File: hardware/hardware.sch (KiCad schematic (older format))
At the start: 18 parts, among them J1 USB_B_Micro, U1 USBLC6-2, U2 PIC18F45K50_QFP, U3 LM317A, U4 DW01+G, U5 TP4056

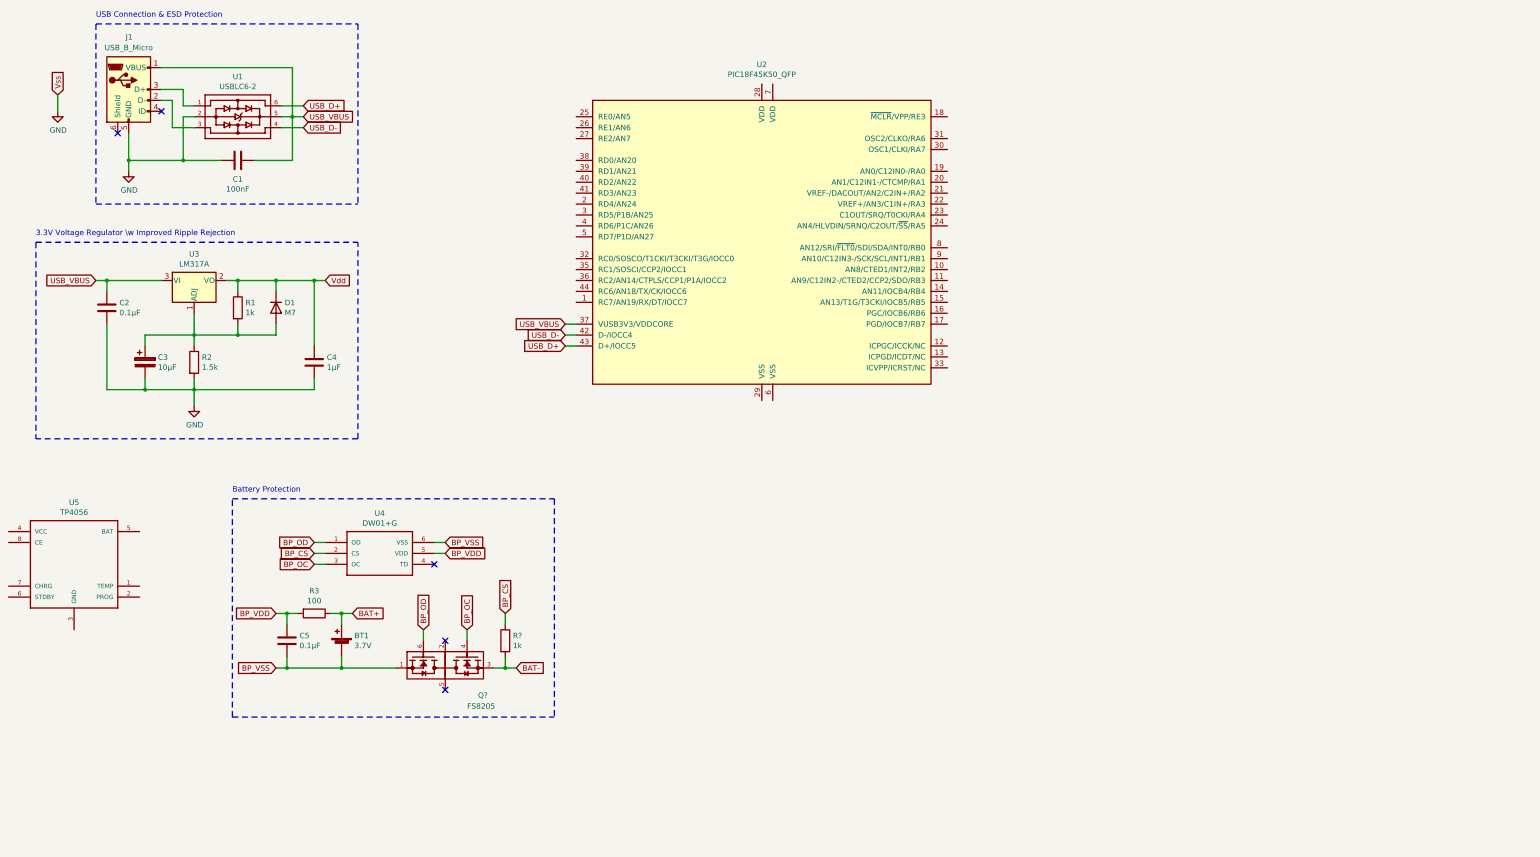
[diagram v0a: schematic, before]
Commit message: Battery management circuit.
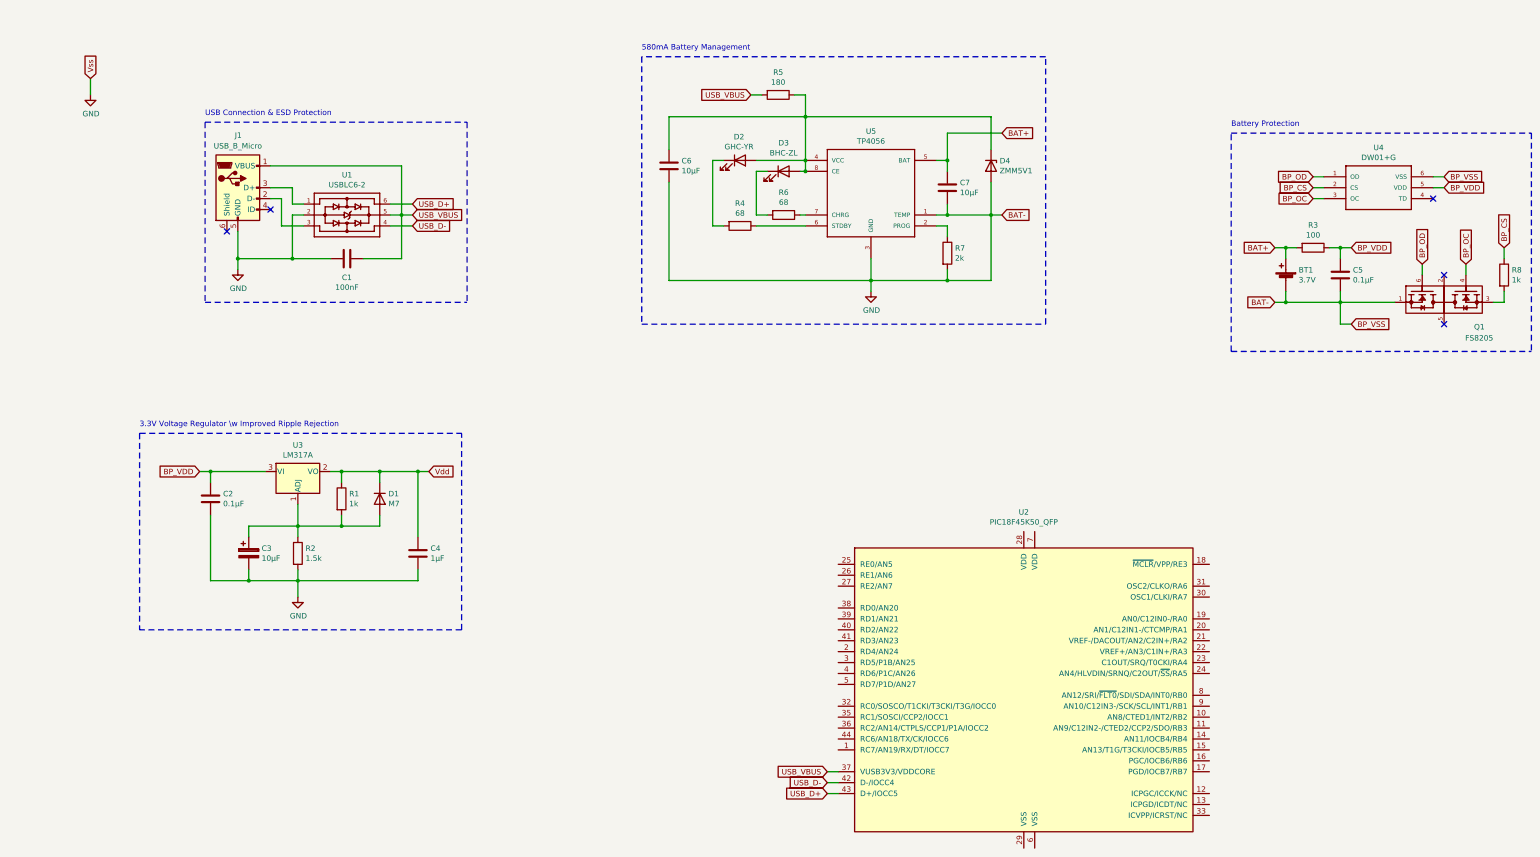
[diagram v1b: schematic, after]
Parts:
- added C6, C7: 10μF, symbol Device:C
- added D2: GHC-YR, symbol Device:LED
- added D3: BHC-ZL, symbol Device:LED
- added D4: ZMM5V1, Diode_SMD:D_MiniMELF_Handsoldering, symbol Device:D_Zener
- added R4, R6: 68, symbol Device:R
- added R5: 180, symbol Device:R
- added R7: 2k, symbol Device:R
- gave numbers to parts that had none: 2
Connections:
- net BP_VSS is gone; now on net GND: BT1.2 (-), C5.2, Q1.1, U4.6 (VSS)
- net BAT+: now also R3.2, U5.5 (BAT), C7.1; no longer R3.1
- net BP_VDD: now also C2.1, R3.1, U3.3 (VI); no longer R3.2
- net GND: now also U5.1 (TEMP), U5.3 (GND), C6.2, C7.2, D4.2 (A), R7.2
- net USB_VBUS: now also R5.2; no longer C2.1, U3.3 (VI)
- net at U5.2 (PROG): now also R7.1
- net at U5.4 (VCC): now also U5.8 (CE), C6.1, D2.2 (A), D3.2 (A), D4.1 (K), R5.1
- net at U5.6 (STDBY): now also R4.1
- net at U5.7 (CHRG): now also R6.1
- net BAT-: no longer names the net of Q1.3, R8.2
- new net: D2.1 (K), R4.2
- new net: D3.1 (K), R6.2
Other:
- note added: "580mA Battery Management"
- moved on the sheet: BT1, C1, C2, C3, C4, C5, D1, J1, Q1, R1, R2, R3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
